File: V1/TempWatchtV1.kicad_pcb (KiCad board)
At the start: 4 copper layers, 70 x 35 mm, 65 parts, among them CN1 SM03B-SRSS-TB(LF)(SN)(P), CN10 SM04B-SRSS-TB (LF)(SN), CN11 SM02B-PASS-1-TBT(LF)(SN), CN2 SM03B-SRSS-TB(LF)(SN)(P), CN3 SM03B-SRSS-TB(LF)(SN)(P), CN4 SM03B-SRSS-TB(LF)(SN)(P), CN5 SM03B-SRSS-TB(LF)(SN)(P), CN6 SM03B-SRSS-TB(LF)(SN)(P), CN7 SM03B-SRSS-TB(LF)(SN)(P), CN8 SM03B-SRSS-TB(LF)(SN)(P), Q1 BC817-25Q-7-F, Q2 BC817-25Q-7-F, SW1 KH-6X6X5H-STM, SW2 KH-6X6X5H-STM, U1 MCP2515-I/ST, U2 SN65HVD230D, U4 ESP32-S3-WROOM-1(N8R2), U5 YTC-TC16S-24, U6 CP2102N-A02-GQFN28R, U7 TPS82130SILR, U9 H7651-33PR, X2 10MHz

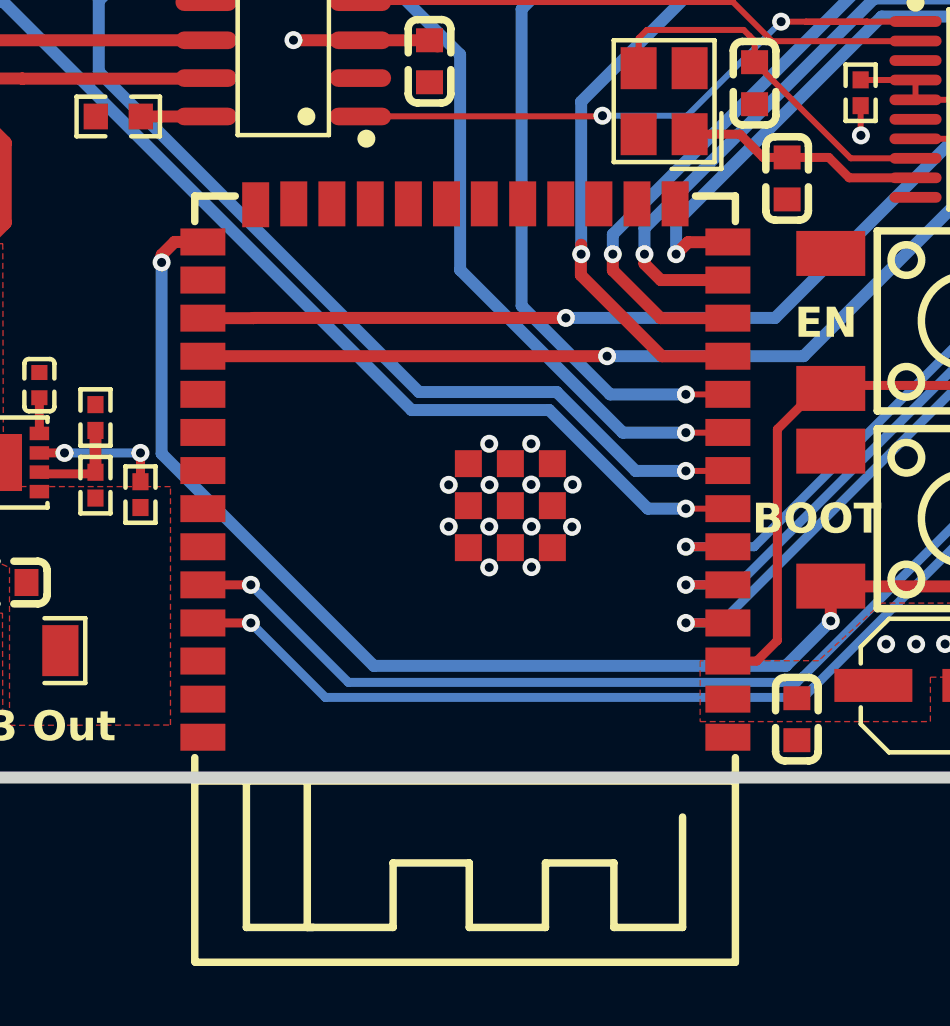
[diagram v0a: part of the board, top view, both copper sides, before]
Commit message: Latest
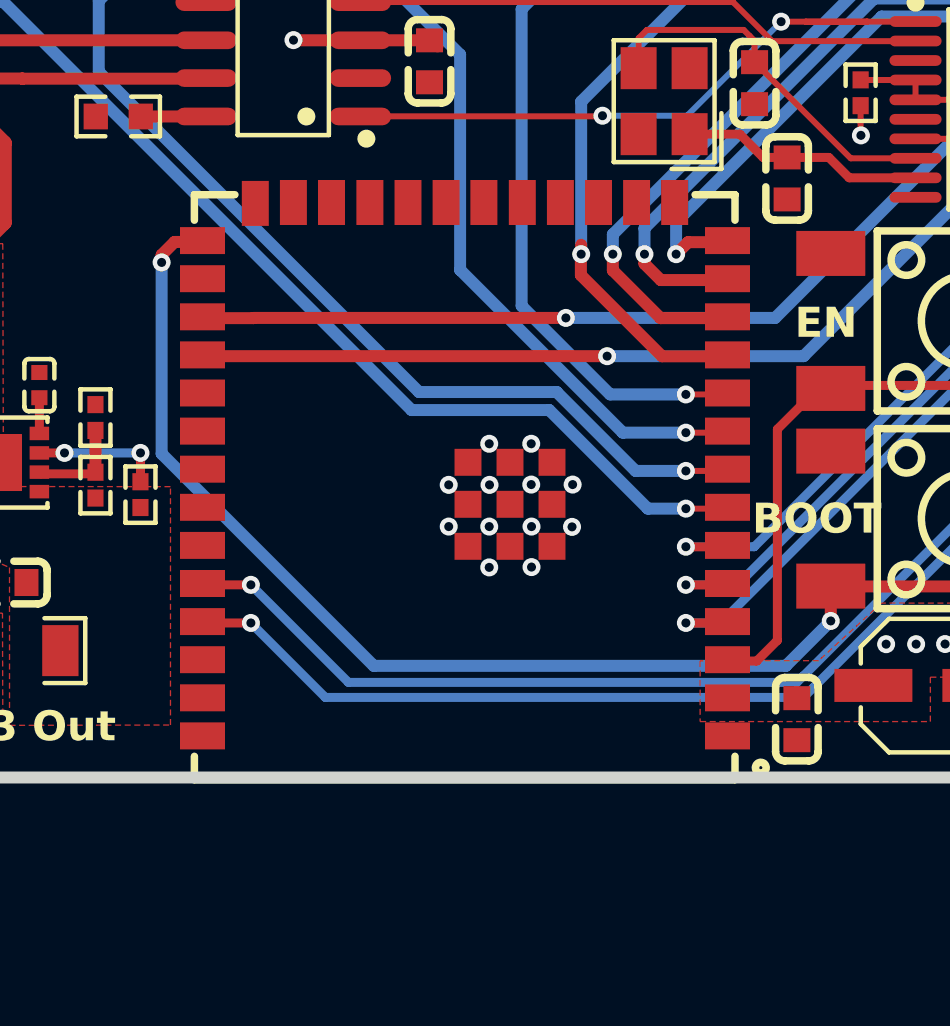
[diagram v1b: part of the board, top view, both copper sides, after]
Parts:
- removed U4: ESP32-S3-WROOM-1(N8R2), easyeda2kicad:WIRELM-SMD_ESP32-S3-WROOM-1
- added U3: ESP32-S3-WROOM-1U-N8R2, easyeda2kicad:WIRELM-SMD_ESP32-S3-WROOM-1U, F.Cu at (131.8, 114.7)
